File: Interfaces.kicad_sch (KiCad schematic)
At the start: 6 parts, among them J6 I/O_Headers_1

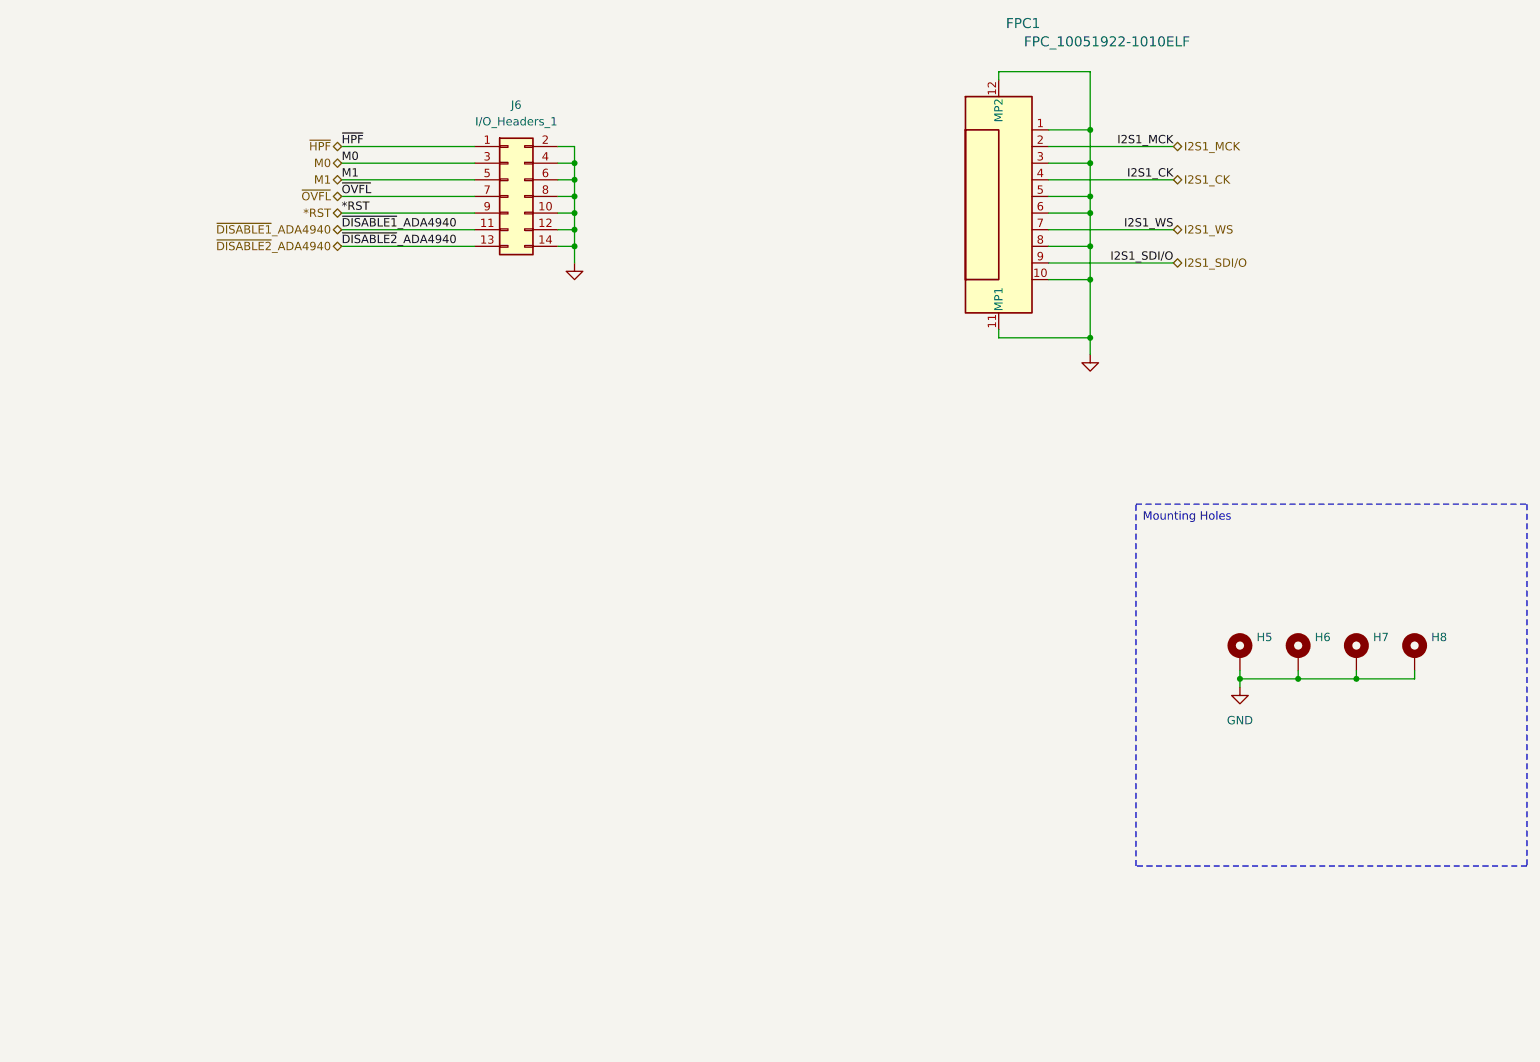
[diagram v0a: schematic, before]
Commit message: Update
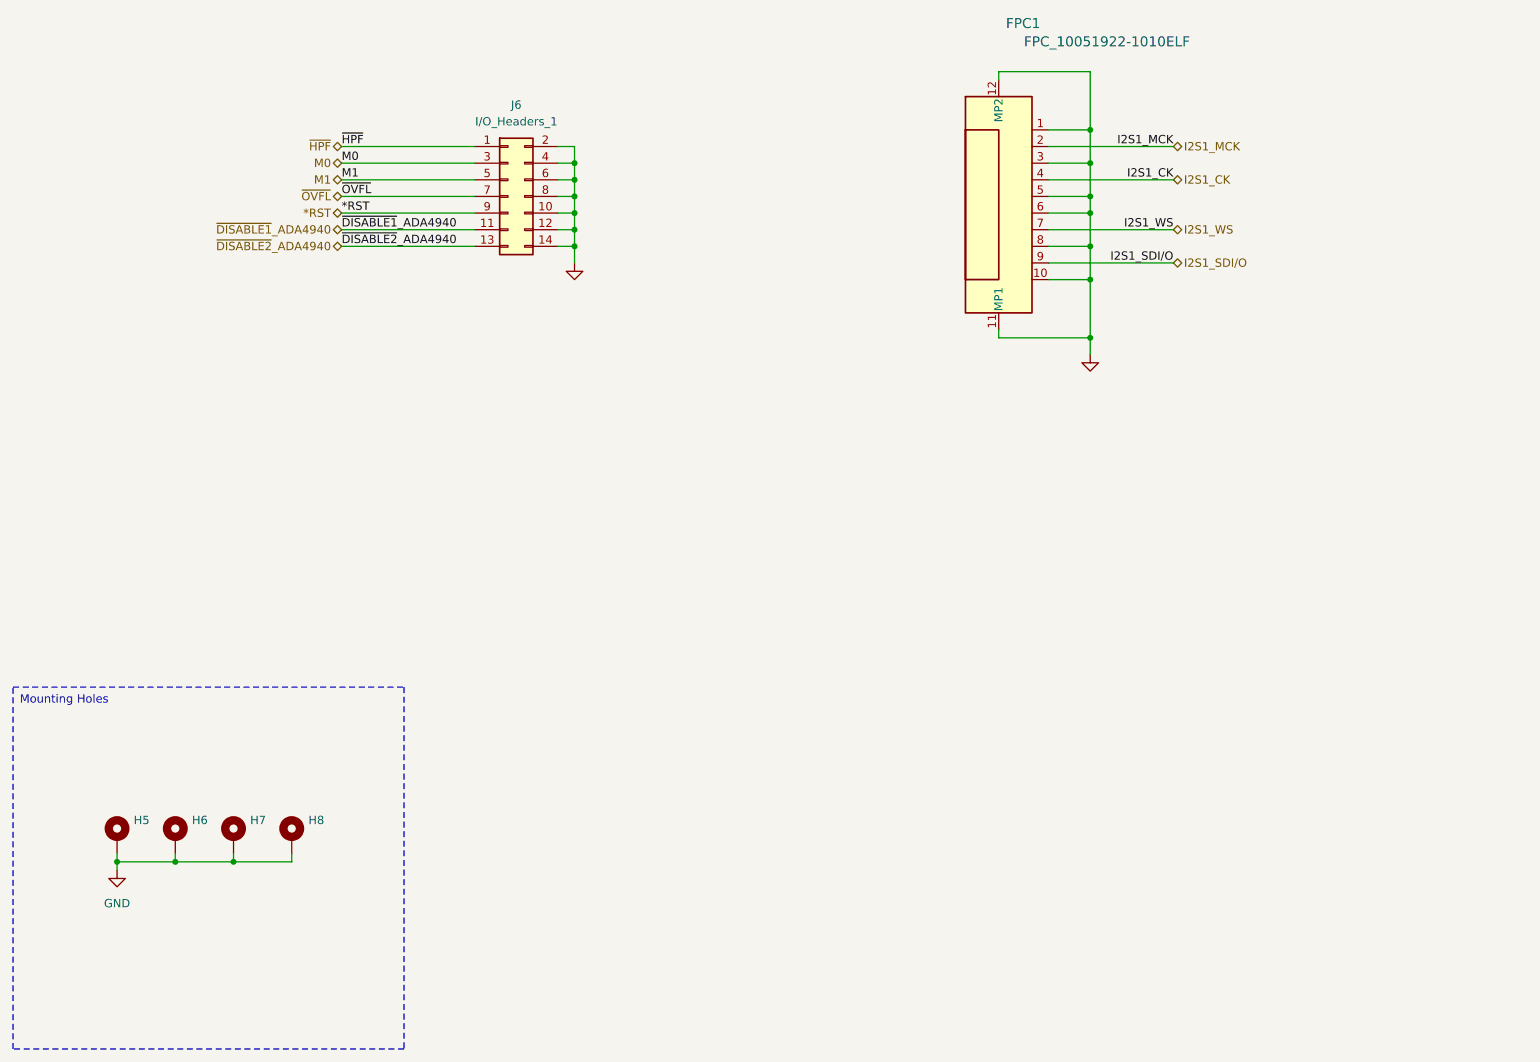
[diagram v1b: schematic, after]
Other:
- moved on the sheet: H5, H6, H7, H8
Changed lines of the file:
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@@
 	)
 	(junction
-		(at 223.52 135.89)
+		(at 52.07 163.83)
 		(diameter 0)
 		(color 0 0 0 0)
 	)
 	(junction
-		(at 214.63 135.89)
+		(at 43.18 163.83)
 		(diameter 0)
 		(color 0 0 0 0)
@@
 	)
 	(junction
-		(at 232.41 135.89)
+		(at 60.96 163.83)
 		(diameter 0)
 		(color 0 0 0 0)
@@
 	(wire
 		(pts
-			(xy 223.52 135.89) (xy 214.63 135.89)
+			(xy 52.07 163.83) (xy 43.18 163.83)
 		)
 		(stroke
@@
 	(wire
 		(pts
-			(xy 214.63 135.89) (xy 214.63 137.16)
+			(xy 43.18 163.83) (xy 43.18 165.1)
 		)
 		(stroke
@@
 	(wire
 		(pts
-			(xy 241.3 135.89) (xy 232.41 135.89)
+			(xy 69.85 163.83) (xy 60.96 163.83)
 		)
 		(stroke
@@
 	(wire
 		(pts
-			(xy 223.52 134.62) (xy 223.52 135.89)
+			(xy 52.07 162.56) (xy 52.07 163.83)
 		)
 		(stroke
@@
 	(wire
 		(pts
-			(xy 232.41 135.89) (xy 223.52 135.89)
-		)
-		(stroke
-			(width 0)
-			(type default)
-		)
-	)
-	(wire
-		(pts
-			(xy 214.63 134.62) (xy 214.63 135.89)
+			(xy 60.96 163.83) (xy 52.07 163.83)
+		)
+		(stroke
+			(width 0)
+			(type default)
+		)
+	)
+	(wire
+		(pts
+			(xy 43.18 162.56) (xy 43.18 163.83)
 		)
 		(stroke
@@
 	(wire
 		(pts
-			(xy 241.3 134.62) (xy 241.3 135.89)
+			(xy 69.85 162.56) (xy 69.85 163.83)
 		)
 		(stroke
@@
 	(wire
 		(pts
-			(xy 232.41 134.62) (xy 232.41 135.89)
+			(xy 60.96 162.56) (xy 60.96 163.83)
 		)
 		(stroke
@@
 	(text_box "Mounting Holes"
 		(exclude_from_sim no)
-		(at 198.755 109.22 0)
+		(at 27.305 137.16 0)
 		(size 59.69 55.245)
 		(stroke
@@
 	(symbol
 		(lib_id "Mechanical:MountingHole_Pad")
-		(at 232.41 132.08 0)
+		(at 60.96 160.02 0)
 		(unit 1)
 		(exclude_from_sim yes)
@@
 		(fields_autoplaced yes)
 		(property "Reference" "H7"
-			(at 234.95 129.5399 0)
+			(at 63.5 157.4799 0)
 			(effects
 				(font
@@
 		)
 		(property "Value" "MountingHole_Pad"
-			(at 234.95 132.0799 0)
+			(at 63.5 160.0199 0)
 			(effects
 				(font
@@
 		)
 		(property "Footprint" "MountingHole:MountingHole_3.2mm_M3_Pad"
-			(at 232.41 132.08 0)
+			(at 60.96 160.02 0)
 			(effects
 				(font
@@
 		)
 		(property "Datasheet" "~"
-			(at 232.41 132.08 0)
+			(at 60.96 160.02 0)
 			(effects
 				(font
@@
 		)
 		(property "Description" "Mounting Hole with connection"
-			(at 232.41 132.08 0)
+			(at 60.96 160.02 0)
 			(effects
 				(font
@@
 	(symbol
 		(lib_id "power:GND")
-		(at 214.63 137.16 0)
+		(at 43.18 165.1 0)
 		(unit 1)
 		(exclude_from_sim no)
@@
 		(fields_autoplaced yes)
 		(property "Reference" "#PWR023"
-			(at 214.63 143.51 0)
+			(at 43.18 171.45 0)
 			(effects
 				(font
@@
 		)
 		(property "Value" "GND"
-			(at 214.63 142.24 0)
+			(at 43.18 170.18 0)
 			(effects
 				(font
@@
 		)
 		(property "Footprint" ""
-			(at 214.63 137.16 0)
+			(at 43.18 165.1 0)
 			(effects
 				(font
@@
 		)
 		(property "Datasheet" ""
-			(at 214.63 137.16 0)
+			(at 43.18 165.1 0)
 			(effects
 				(font
@@
 		)
 		(property "Description" "Power symbol creates a global label with name \"GND\" , ground"
-			(at 214.63 137.16 0)
+			(at 43.18 165.1 0)
 			(effects
 				(font
@@
 	(symbol
 		(lib_id "Mechanical:MountingHole_Pad")
-		(at 214.63 132.08 0)
+		(at 43.18 160.02 0)
 		(unit 1)
 		(exclude_from_sim yes)
@@
 		(fields_autoplaced yes)
 		(property "Reference" "H5"
-			(at 217.17 129.5399 0)
+			(at 45.72 157.4799 0)
 			(effects
 				(font
@@
 		)
 		(property "Value" "MountingHole_Pad"
-			(at 217.17 132.0799 0)
+			(at 45.72 160.0199 0)
 			(effects
 				(font
@@
 		)
 		(property "Footprint" "MountingHole:MountingHole_3.2mm_M3_Pad"
-			(at 214.63 132.08 0)
+			(at 43.18 160.02 0)
 			(effects
 				(font
@@
 		)
 		(property "Datasheet" "~"
-			(at 214.63 132.08 0)
+			(at 43.18 160.02 0)
 			(effects
 				(font
@@
 		)
 		(property "Description" "Mounting Hole with connection"
-			(at 214.63 132.08 0)
+			(at 43.18 160.02 0)
 			(effects
 				(font
@@
 	(symbol
 		(lib_id "Mechanical:MountingHole_Pad")
-		(at 241.3 132.08 0)
+		(at 69.85 160.02 0)
 		(unit 1)
 		(exclude_from_sim yes)
@@
 		(fields_autoplaced yes)
 		(property "Reference" "H8"
-			(at 243.84 129.5399 0)
+			(at 72.39 157.4799 0)
 			(effects
 				(font
@@
 		)
 		(property "Value" "MountingHole_Pad"
-			(at 243.84 132.0799 0)
+			(at 72.39 160.0199 0)
 			(effects
 				(font
@@
 		)
 		(property "Footprint" "MountingHole:MountingHole_3.2mm_M3_Pad"
-			(at 241.3 132.08 0)
+			(at 69.85 160.02 0)
 			(effects
 				(font
@@
 		)
 		(property "Datasheet" "~"
-			(at 241.3 132.08 0)
+			(at 69.85 160.02 0)
 			(effects
 				(font
@@
 		)
 		(property "Description" "Mounting Hole with connection"
-			(at 241.3 132.08 0)
+			(at 69.85 160.02 0)
 			(effects
 				(font
@@
 	(symbol
 		(lib_id "Mechanical:MountingHole_Pad")
-		(at 223.52 132.08 0)
+		(at 52.07 160.02 0)
 		(unit 1)
 		(exclude_from_sim yes)
@@
 		(fields_autoplaced yes)
 		(property "Reference" "H6"
-			(at 226.06 129.5399 0)
+			(at 54.61 157.4799 0)
 			(effects
 				(font
@@
 		)
 		(property "Value" "MountingHole_Pad"
-			(at 226.06 132.0799 0)
+			(at 54.61 160.0199 0)
 			(effects
 				(font
@@
 		)
 		(property "Footprint" "MountingHole:MountingHole_3.2mm_M3_Pad"
-			(at 223.52 132.08 0)
+			(at 52.07 160.02 0)
 			(effects
 				(font
@@
 		)
 		(property "Datasheet" "~"
-			(at 223.52 132.08 0)
+			(at 52.07 160.02 0)
 			(effects
 				(font
@@
 		)
 		(property "Description" "Mounting Hole with connection"
-			(at 223.52 132.08 0)
-			(effects
-				(font
+			(at 52.07 160.02 0)
+			(effects
+				(font

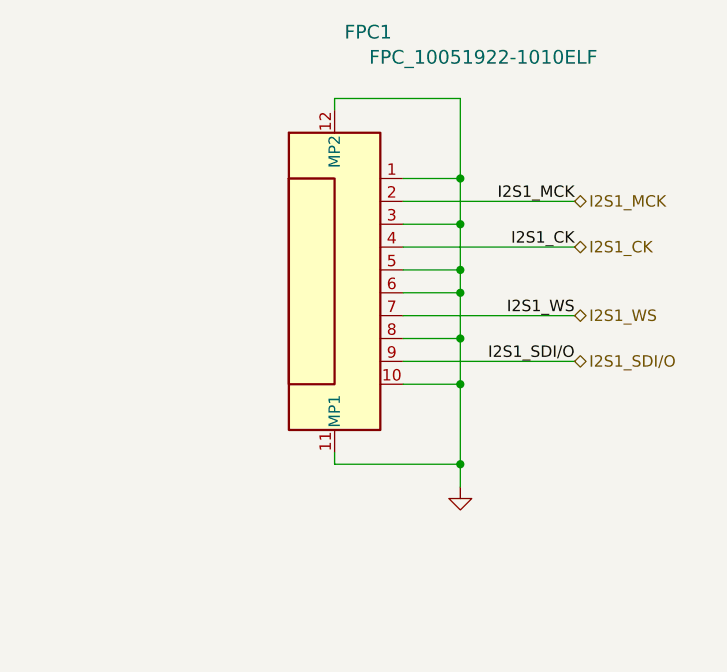
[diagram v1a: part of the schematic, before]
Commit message: Update
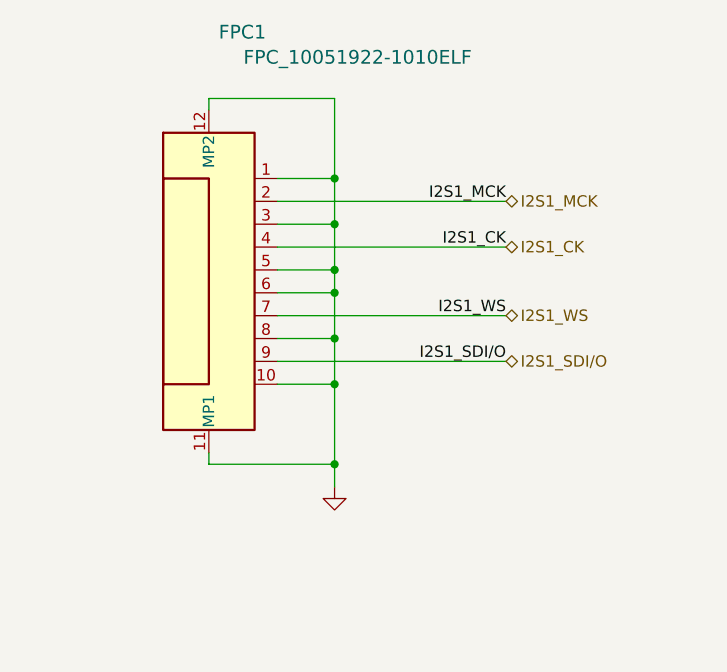
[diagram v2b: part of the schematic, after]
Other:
- moved on the sheet: FPC1
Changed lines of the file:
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@@
 	)
 	(junction
-		(at 191.77 74.93)
+		(at 177.8 74.93)
 		(diameter 0)
 		(color 0 0 0 0)
@@
 	)
 	(junction
-		(at 191.77 64.77)
-		(diameter 0)
-		(color 0 0 0 0)
-	)
-	(junction
-		(at 191.77 83.82)
+		(at 177.8 64.77)
+		(diameter 0)
+		(color 0 0 0 0)
+	)
+	(junction
+		(at 177.8 83.82)
 		(diameter 0)
 		(color 0 0 0 0)
@@
 	)
 	(junction
-		(at 191.77 69.85)
+		(at 177.8 69.85)
 		(diameter 0)
 		(color 0 0 0 0)
@@
 	)
 	(junction
-		(at 191.77 62.23)
-		(diameter 0)
-		(color 0 0 0 0)
-	)
-	(junction
-		(at 191.77 52.07)
-		(diameter 0)
-		(color 0 0 0 0)
-	)
-	(junction
-		(at 191.77 57.15)
-		(diameter 0)
-		(color 0 0 0 0)
-	)
-	(wire
-		(pts
-			(xy 185.42 59.69) (xy 204.47 59.69)
-		)
-		(stroke
-			(width 0)
-			(type default)
-		)
-	)
-	(wire
-		(pts
-			(xy 177.8 43.18) (xy 191.77 43.18)
+		(at 177.8 62.23)
+		(diameter 0)
+		(color 0 0 0 0)
+	)
+	(junction
+		(at 177.8 52.07)
+		(diameter 0)
+		(color 0 0 0 0)
+	)
+	(junction
+		(at 177.8 57.15)
+		(diameter 0)
+		(color 0 0 0 0)
+	)
+	(wire
+		(pts
+			(xy 171.45 59.69) (xy 196.85 59.69)
+		)
+		(stroke
+			(width 0)
+			(type default)
+		)
+	)
+	(wire
+		(pts
+			(xy 163.83 43.18) (xy 177.8 43.18)
 		)
 		(stroke
@@
 	(wire
 		(pts
-			(xy 185.42 72.39) (xy 204.47 72.39)
+			(xy 171.45 72.39) (xy 196.85 72.39)
 		)
 		(stroke
@@
 	(wire
 		(pts
-			(xy 185.42 74.93) (xy 191.77 74.93)
+			(xy 171.45 74.93) (xy 177.8 74.93)
 		)
 		(stroke
@@
 	(wire
 		(pts
-			(xy 177.8 82.55) (xy 177.8 83.82)
-		)
-		(stroke
-			(width 0)
-			(type default)
-		)
-	)
-	(wire
-		(pts
-			(xy 185.42 62.23) (xy 191.77 62.23)
+			(xy 163.83 82.55) (xy 163.83 83.82)
+		)
+		(stroke
+			(width 0)
+			(type default)
+		)
+	)
+	(wire
+		(pts
+			(xy 171.45 62.23) (xy 177.8 62.23)
 		)
 		(stroke
@@
 	(wire
 		(pts
-			(xy 191.77 52.07) (xy 191.77 57.15)
-		)
-		(stroke
-			(width 0)
-			(type default)
-		)
-	)
-	(wire
-		(pts
-			(xy 191.77 57.15) (xy 191.77 62.23)
-		)
-		(stroke
-			(width 0)
-			(type default)
-		)
-	)
-	(wire
-		(pts
-			(xy 177.8 44.45) (xy 177.8 43.18)
+			(xy 177.8 52.07) (xy 177.8 57.15)
+		)
+		(stroke
+			(width 0)
+			(type default)
+		)
+	)
+	(wire
+		(pts
+			(xy 177.8 57.15) (xy 177.8 62.23)
+		)
+		(stroke
+			(width 0)
+			(type default)
+		)
+	)
+	(wire
+		(pts
+			(xy 163.83 44.45) (xy 163.83 43.18)
 		)
 		(stroke
@@
 	(wire
 		(pts
-			(xy 191.77 64.77) (xy 191.77 69.85)
+			(xy 177.8 64.77) (xy 177.8 69.85)
 		)
 		(stroke
@@
 	(wire
 		(pts
-			(xy 191.77 62.23) (xy 191.77 64.77)
+			(xy 177.8 62.23) (xy 177.8 64.77)
 		)
 		(stroke
@@
 	(wire
 		(pts
-			(xy 185.42 69.85) (xy 191.77 69.85)
+			(xy 171.45 69.85) (xy 177.8 69.85)
 		)
 		(stroke
@@
 	(wire
 		(pts
-			(xy 185.42 54.61) (xy 204.47 54.61)
-		)
-		(stroke
-			(width 0)
-			(type default)
-		)
-	)
-	(wire
-		(pts
-			(xy 185.42 64.77) (xy 191.77 64.77)
+			(xy 171.45 54.61) (xy 196.85 54.61)
+		)
+		(stroke
+			(width 0)
+			(type default)
+		)
+	)
+	(wire
+		(pts
+			(xy 171.45 64.77) (xy 177.8 64.77)
 		)
 		(stroke
@@
 	(wire
 		(pts
-			(xy 177.8 83.82) (xy 191.77 83.82)
-		)
-		(stroke
-			(width 0)
-			(type default)
-		)
-	)
-	(wire
-		(pts
-			(xy 191.77 83.82) (xy 191.77 86.36)
+			(xy 163.83 83.82) (xy 177.8 83.82)
+		)
+		(stroke
+			(width 0)
+			(type default)
+		)
+	)
+	(wire
+		(pts
+			(xy 177.8 83.82) (xy 177.8 86.36)
 		)
 		(stroke
@@
 	(wire
 		(pts
-			(xy 185.42 67.31) (xy 204.47 67.31)
+			(xy 171.45 67.31) (xy 196.85 67.31)
 		)
 		(stroke
@@
 	(wire
 		(pts
-			(xy 185.42 52.07) (xy 191.77 52.07)
-		)
-		(stroke
-			(width 0)
-			(type default)
-		)
-	)
-	(wire
-		(pts
-			(xy 191.77 69.85) (xy 191.77 74.93)
+			(xy 171.45 52.07) (xy 177.8 52.07)
+		)
+		(stroke
+			(width 0)
+			(type default)
+		)
+	)
+	(wire
+		(pts
+			(xy 177.8 69.85) (xy 177.8 74.93)
 		)
 		(stroke
@@
 	(wire
 		(pts
-			(xy 185.42 57.15) (xy 191.77 57.15)
+			(xy 171.45 57.15) (xy 177.8 57.15)
 		)
 		(stroke
@@
 	(wire
 		(pts
-			(xy 191.77 43.18) (xy 191.77 52.07)
+			(xy 177.8 43.18) (xy 177.8 52.07)
 		)
 		(stroke
@@
 	(wire
 		(pts
-			(xy 191.77 74.93) (xy 191.77 83.82)
+			(xy 177.8 74.93) (xy 177.8 83.82)
 		)
 		(stroke
@@
 	)
 	(label "I2S1_SDI{slash}O"
-		(at 204.47 72.39 180)
+		(at 196.85 72.39 180)
 		(fields_autoplaced yes)
 		(effects
@@
 	)
 	(label "I2S1_WS"
-		(at 204.47 67.31 180)
+		(at 196.85 67.31 180)
 		(fields_autoplaced yes)
 		(effects
@@
 	)
 	(label "I2S1_CK"
-		(at 204.47 59.69 180)
+		(at 196.85 59.69 180)
 		(fields_autoplaced yes)
 		(effects
@@
 	)
 	(label "I2S1_MCK"
-		(at 204.47 54.61 180)
+		(at 196.85 54.61 180)
 		(fields_autoplaced yes)
 		(effects
@@
 	(hierarchical_label "I2S1_WS"
 		(shape bidirectional)
-		(at 204.47 67.31 0)
+		(at 196.85 67.31 0)
 		(fields_autoplaced yes)
 		(effects
@@
 	(hierarchical_label "I2S1_MCK"
 		(shape bidirectional)
-		(at 204.47 54.61 0)
+		(at 196.85 54.61 0)
 		(fields_autoplaced yes)
 		(effects
@@
 	(hierarchical_label "I2S1_CK"
 		(shape bidirectional)
-		(at 204.47 59.69 0)
+		(at 196.85 59.69 0)
 		(fields_autoplaced yes)
 		(effects
@@
 	(hierarchical_label "I2S1_SDI{slash}O"
 		(shape bidirectional)
-		(at 204.47 72.39 0)
+		(at 196.85 72.39 0)
 		(fields_autoplaced yes)
 		(effects
@@
 	(symbol
 		(lib_id "power:GND")
-		(at 191.77 86.36 0)
+		(at 177.8 86.36 0)
 		(unit 1)
 		(exclude_from_sim no)
@@
 		(dnp no)
 		(property "Reference" "#PWR043"
-			(at 191.77 92.71 0)
+			(at 177.8 92.71 0)
 			(effects
 				(font
@@
 		)
 		(property "Value" "GND"
-			(at 189.23 89.408 90)
+			(at 175.26 89.408 90)
 			(effects
 				(font
@@
 		)
 		(property "Footprint" ""
-			(at 191.77 86.36 0)
+			(at 177.8 86.36 0)
 			(effects
 				(font
@@
 		)
 		(property "Datasheet" ""
-			(at 191.77 86.36 0)
+			(at 177.8 86.36 0)
 			(effects
 				(font
@@
 		)
 		(property "Description" "Power symbol creates a global label with name \"GND\" , ground"
-			(at 191.77 86.36 0)
+			(at 177.8 86.36 0)
 			(effects
 				(font
@@
 	(symbol
 		(lib_id "Personal_Projects:FPC_10051922-1010ELF")
-		(at 172.72 52.07 0)
+		(at 158.75 52.07 0)
 		(unit 1)
 		(exclude_from_sim no)
@@
 		(dnp no)
 		(property "Reference" "FPC1"
-			(at 184.15 35.814 0)
+			(at 170.18 35.814 0)
 			(effects
 				(font
@@
 		)
 		(property "Value" "FPC_10051922-1010ELF"
-			(at 207.01 38.608 0)
+			(at 193.04 38.608 0)
 			(effects
 				(font
@@
 		)
 		(property "Footprint" "Personal_Project:FPC_10051922_1010"
-			(at 172.72 99.06 0)
+			(at 158.75 99.06 0)
 			(effects
 				(font
@@
 		)
 		(property "Datasheet" "10051922-1010ELF"
-			(at 172.72 95.25 0)
+			(at 158.75 95.25 0)
 			(effects
 				(font
@@
 		)
 		(property "Description" ""
-			(at 185.42 52.07 0)
-			(effects
-				(font
+			(at 171.45 52.07 0)
+			(effects
+				(font
